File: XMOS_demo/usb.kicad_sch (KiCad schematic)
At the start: 11 parts, among them J2 USB_C_Receptacle_USB2.0_16P, J4 Screw_Terminal_P3.50mm, U4 TPD3S014

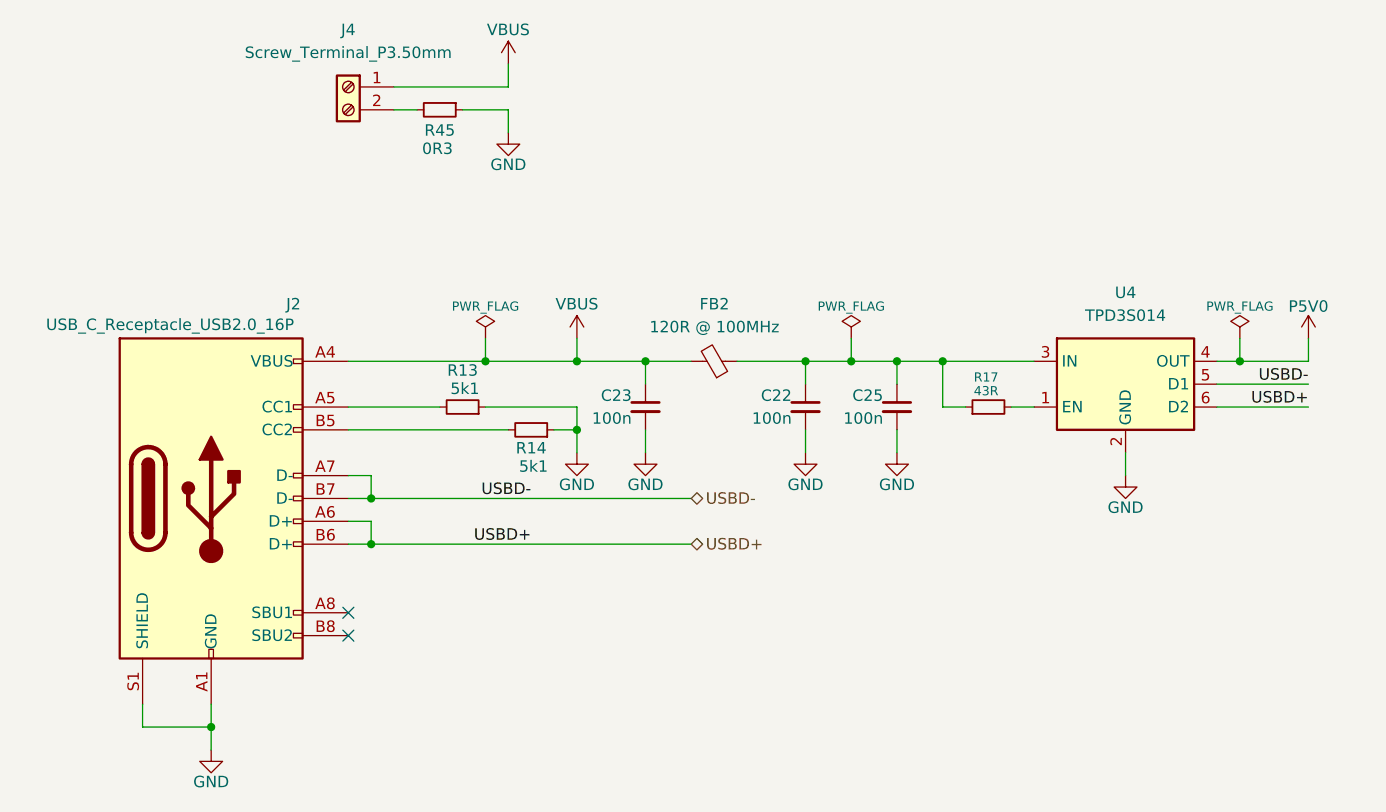
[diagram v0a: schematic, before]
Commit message: sch mostly finished, needs tp, pcb component layout started
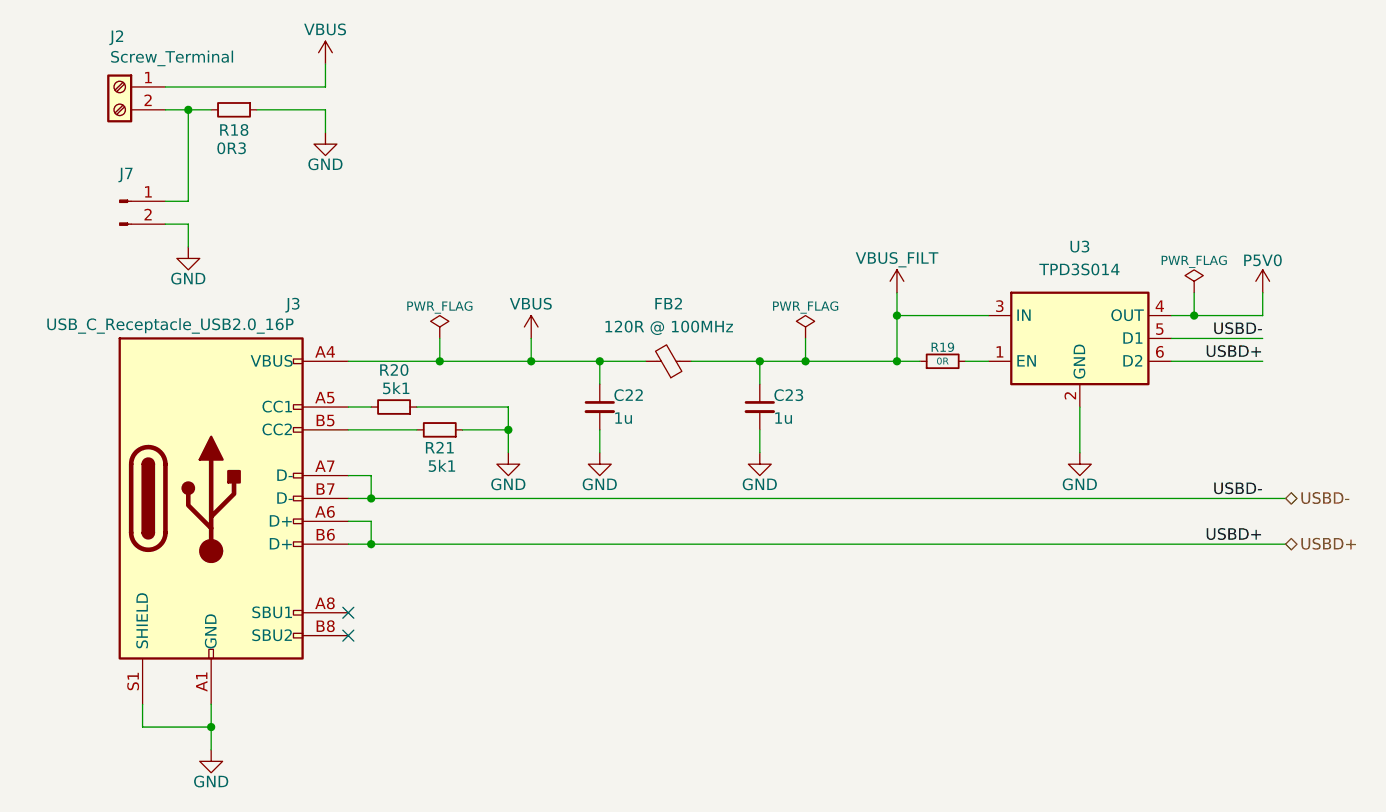
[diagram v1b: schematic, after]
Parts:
- removed C25: 100n, Capacitor_SMD:C_0603_1608Metric, symbol Device:C_Small
- removed R17: 43R, Resistor_SMD:R_0603_1608Metric, symbol Device:R_Small
- added J7: Conn_01x02_Pin, Connector_PinHeader_2.54mm:PinHeader_1x02_P2.54mm_Vertical, symbol Connector:Conn_01x02_Pin
- added R19: 0R, Resistor_SMD:R_0603_1608Metric, symbol Device:R_Small
- C22, C23: value 100n -> 1u
- J2: renamed from J4; value Screw_Terminal_P3.50mm -> Screw_Terminal
- renumbered J2 to J3, R45 to R18, R13 to R20, R14 to R21, U4 to U3
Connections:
- net GND: now also J7.2 (Pin_2)
- net VBUS: now also C22.1; no longer C23.1
- net VBUS_FILT: now reaches FB2.1, U3.3 (IN)
- net VBUS_FILT: now also C23.1, R19.1; no longer C22.1
- net at J2.2 (Pin_2), R18.2: now also J7.1 (Pin_1)
- net at U3.1 (EN): now also R19.2
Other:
- moved on the sheet: FB2, J2, R18, R20, R21, U3
